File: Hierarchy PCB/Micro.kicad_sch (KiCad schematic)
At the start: 2 parts, among them U9 STM32L476RGTx

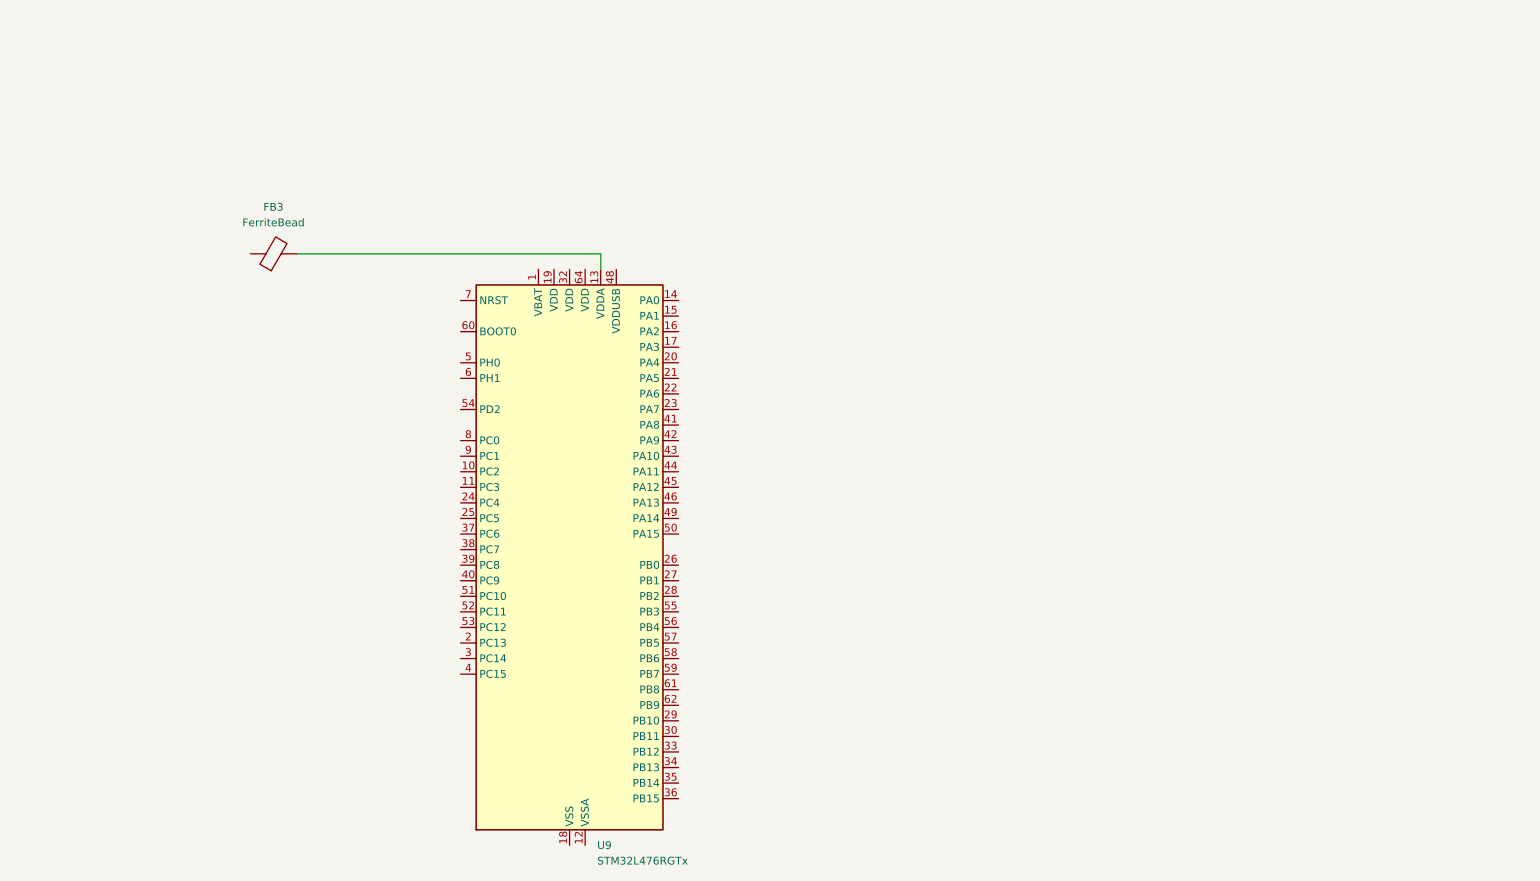
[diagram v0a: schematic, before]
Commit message: Add files via upload
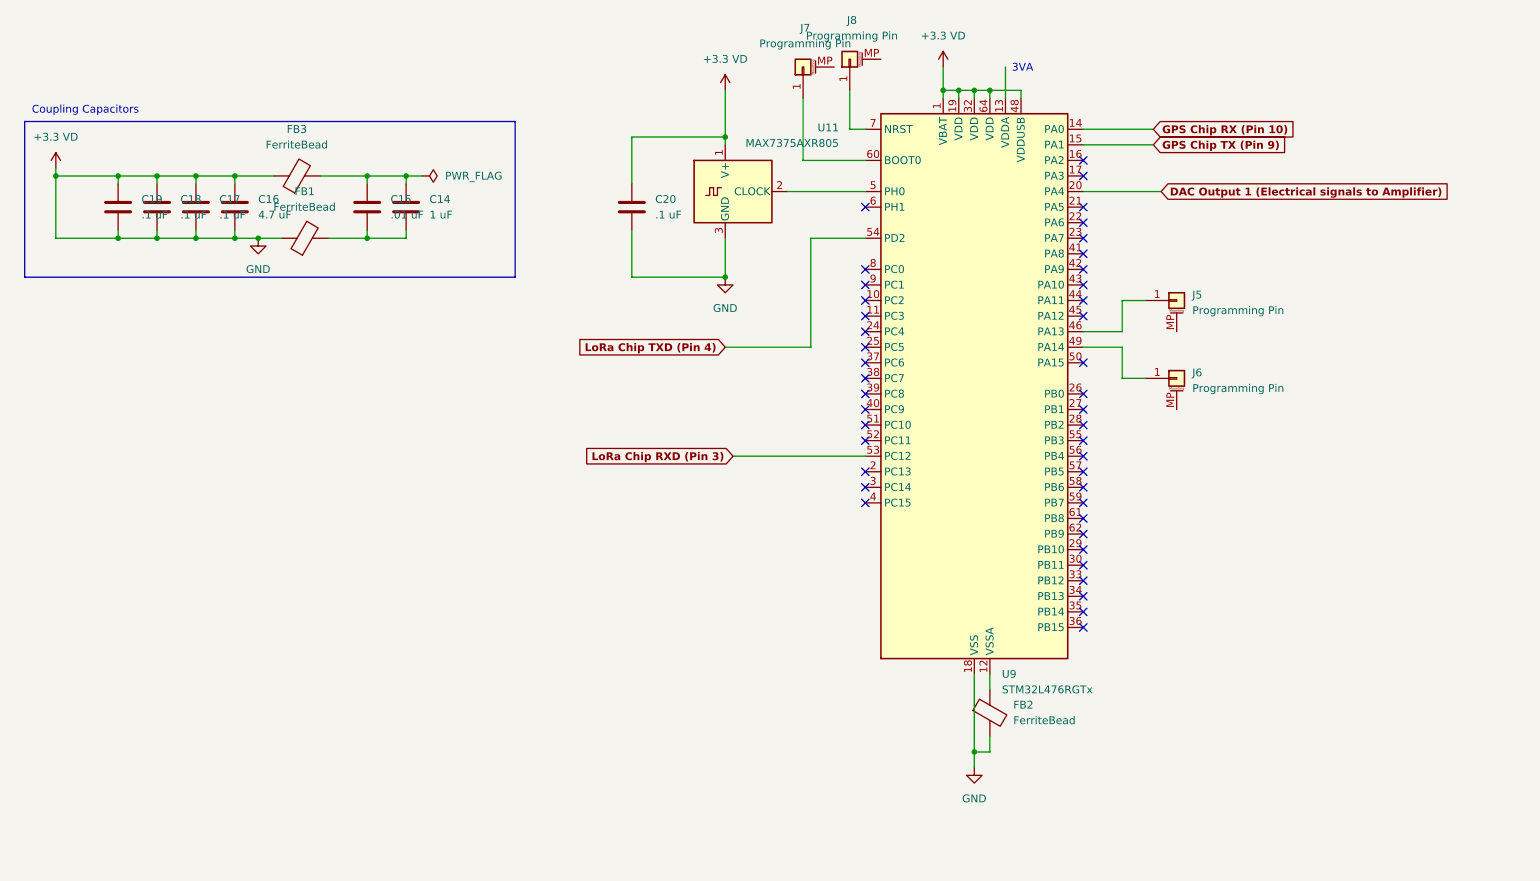
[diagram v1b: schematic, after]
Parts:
- added C14: 1 uF, symbol Device:C
- added C15: .01 uF, symbol Device:C
- added C16: 4.7 uF, symbol Device:C
- added C17, C18, C19, C20: .1 uF, symbol Device:C
- added FB1, FB2: FerriteBead, symbol Device:FerriteBead
- added J5, J6, J7, J8: Programming Pin, symbol Connector_Generic_MountingPin:Conn_01x01_MountingPin
- added U11: MAX7375AXR805, Package_TO_SOT_SMD:SOT-323_SC-70, symbol Oscillator:MAX7375AXR805
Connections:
- net +3.3 VD: now reaches FB3.1
- net +3.3 VD: now also U9.1 (VBAT), U9.18 (VSS), U9.19 (VDD), U9.31 (VSS), U9.32 (VDD), U9.47 (VSS), U9.48 (VDDUSB), U9.63 (VSS), U9.64 (VDD), C16.1, C16.2, C17.1, C17.2, C18.1, C18.2, C19.1, C19.2, C20.1, C20.2, FB1.1, FB2.2, U11.1 (V+), U11.3 (GND)
- net at FB3.2: now also C14.1, C15.1; no longer U9.13 (VDDA)
- net at U9.12 (VSSA): now also FB2.1
- net GPS Chip RX (Pin 10): now reaches U9.14 (PA0)
- net GPS Chip TX (Pin 9): now reaches U9.15 (PA1)
- net DAC Output 1 (Electrical signals to Amplifier): now reaches U9.20 (PA4)
- net at U9.46 (PA13): now also J5.1 (Pin_1)
- net at U9.49 (PA14): now also J6.1 (Pin_1)
- net at U9.5 (PH0): now also U11.2 (CLOCK)
- net LoRa Chip RXD (Pin 3): now reaches U9.53 (PC12)
- net LoRa Chip TXD (Pin 4): now reaches U9.54 (PD2)
- net at U9.60 (BOOT0): now also J7.1 (Pin_1)
- net at U9.7 (NRST): now also J8.1 (Pin_1)
- new net: C14.2, C15.2, FB1.2
- no-connect marks 0 -> 43
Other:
- note added: "3VA"
- note added: "Coupling Capacitors"
- moved on the sheet: FB3, U9
